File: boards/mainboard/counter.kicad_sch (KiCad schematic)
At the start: 8 parts, among them U12 7404, U15 74163, U16 74163, U17 74163

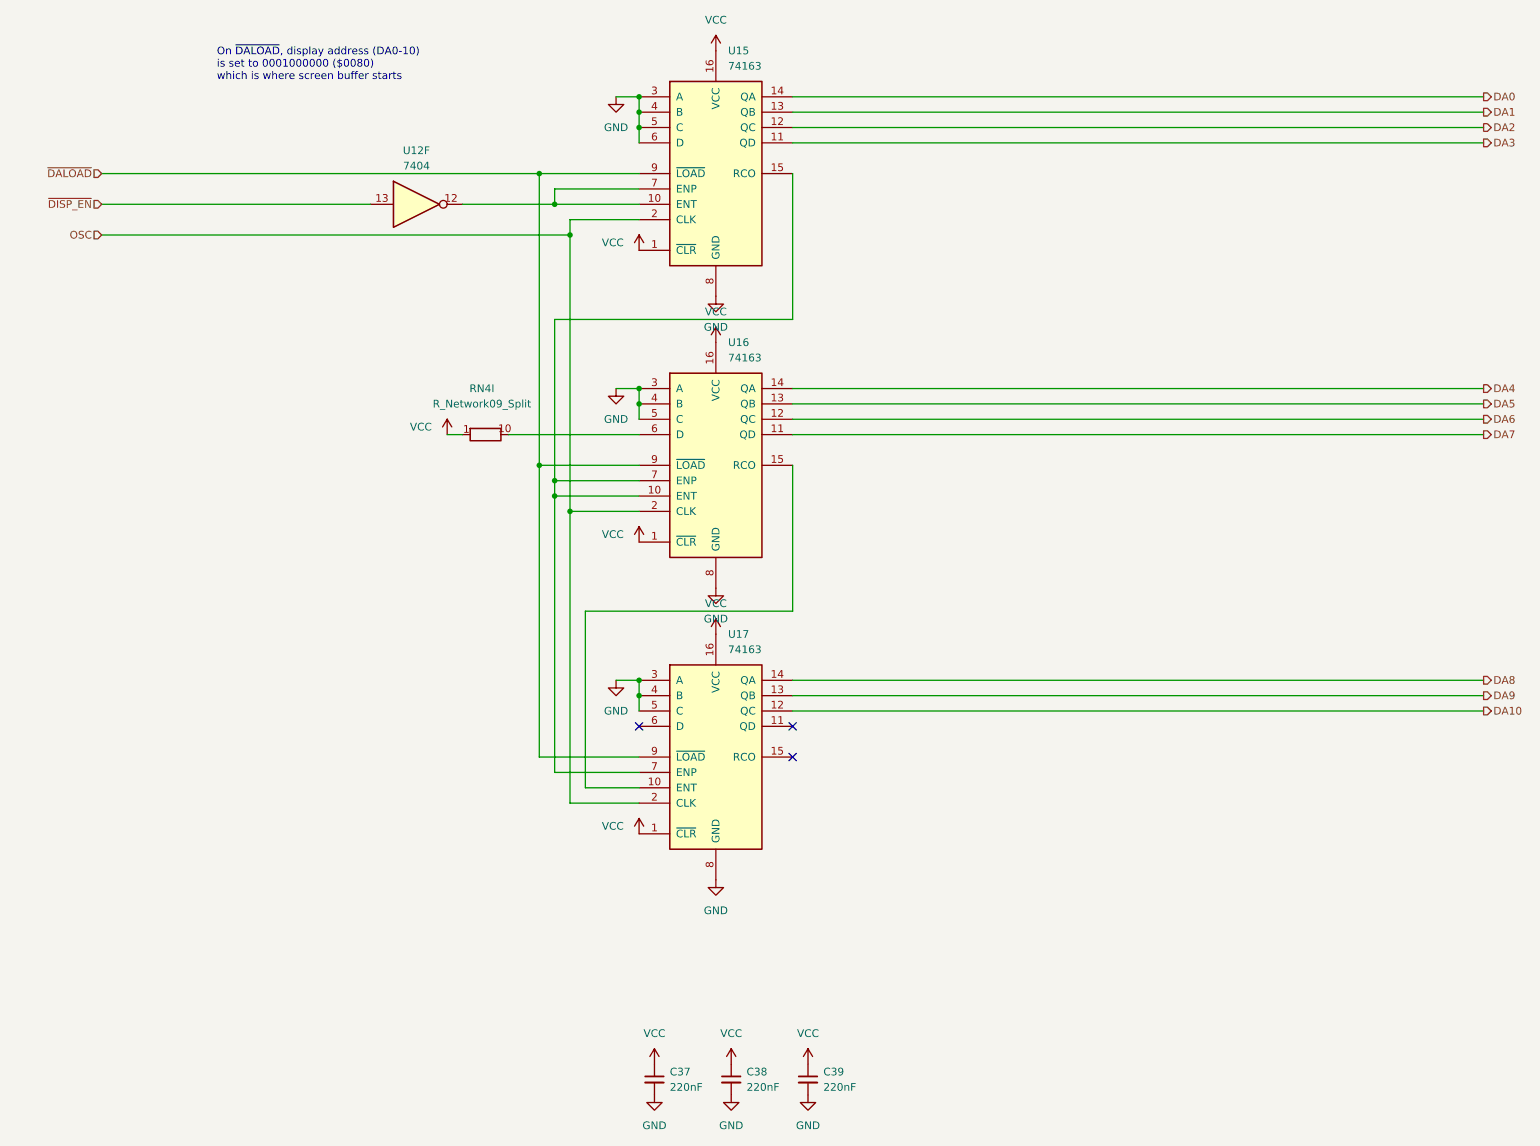
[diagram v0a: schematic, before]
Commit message: organize mainboard schematic
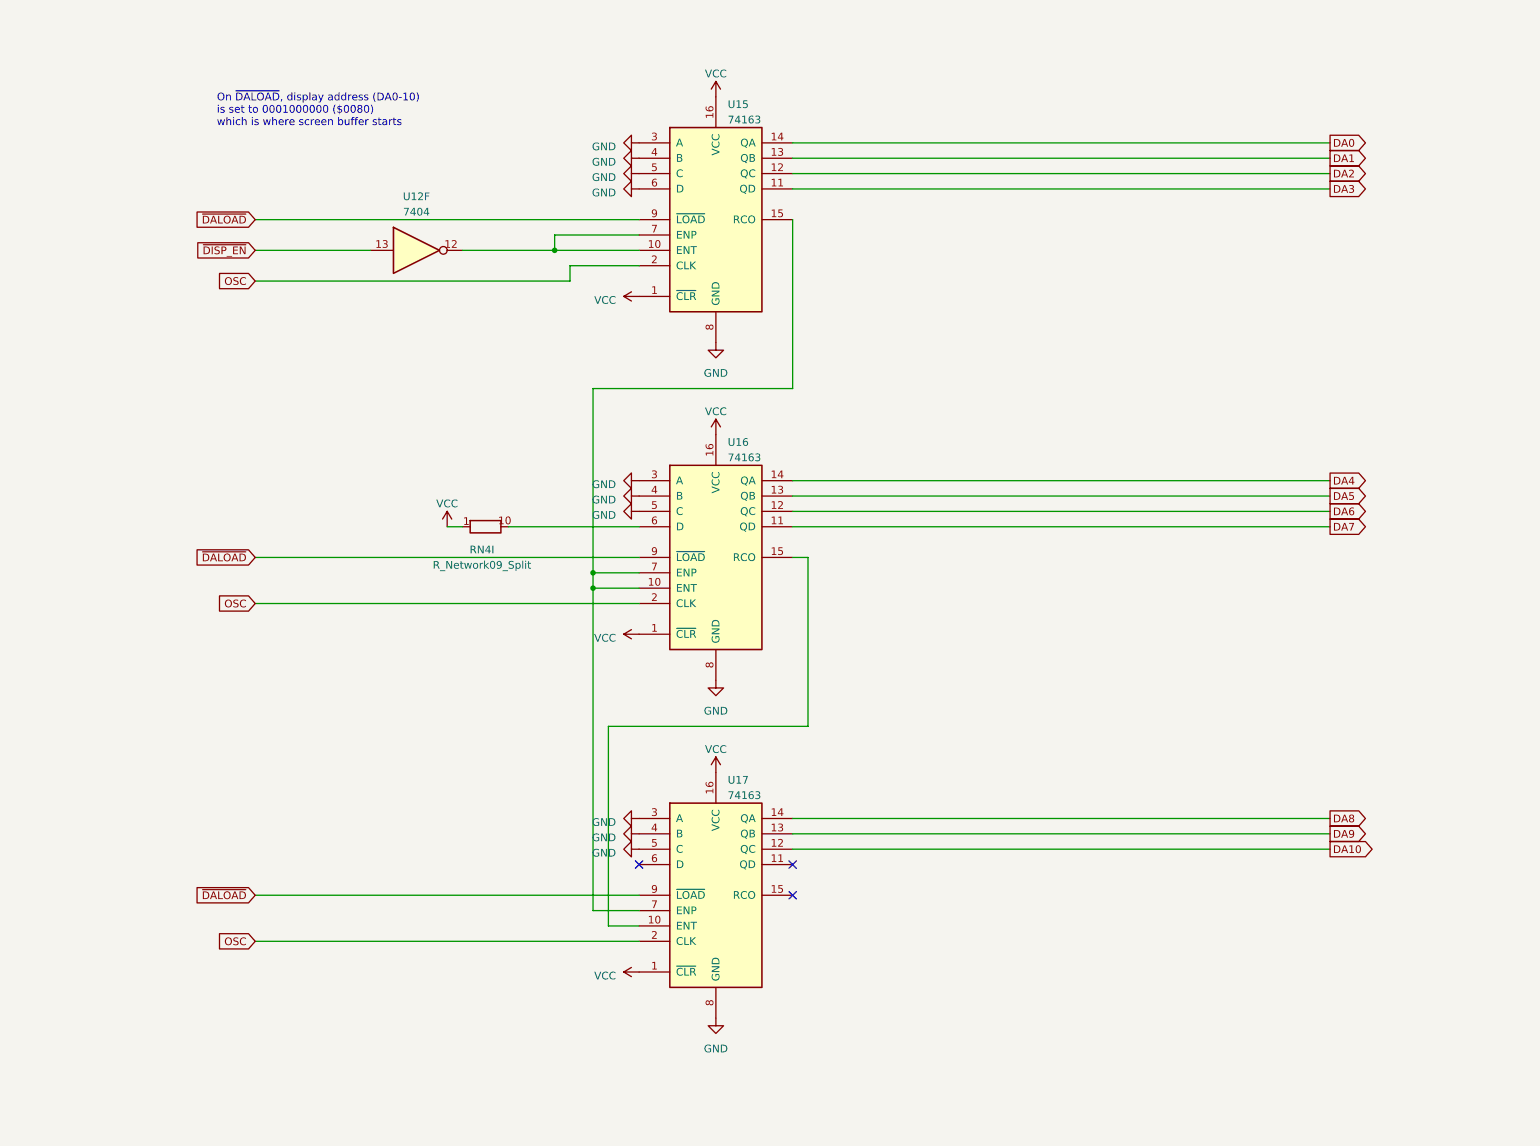
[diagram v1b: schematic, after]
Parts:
- removed C37, C38, C39: 220nF, ambassador:C_Disc_D4.3mm_W1.9mm_P6.35mm, symbol Device:C_Small
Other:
- moved on the sheet: RN4I, U12F, U15, U16, U17
